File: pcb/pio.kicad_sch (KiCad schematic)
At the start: 32 parts, among them J11 GPA[0..3], J4 GPB[0..3], J5 GPB[4..7], J6 BTN[0..3], J7 GPA[4..7], U4 MCP23017T-E/ML

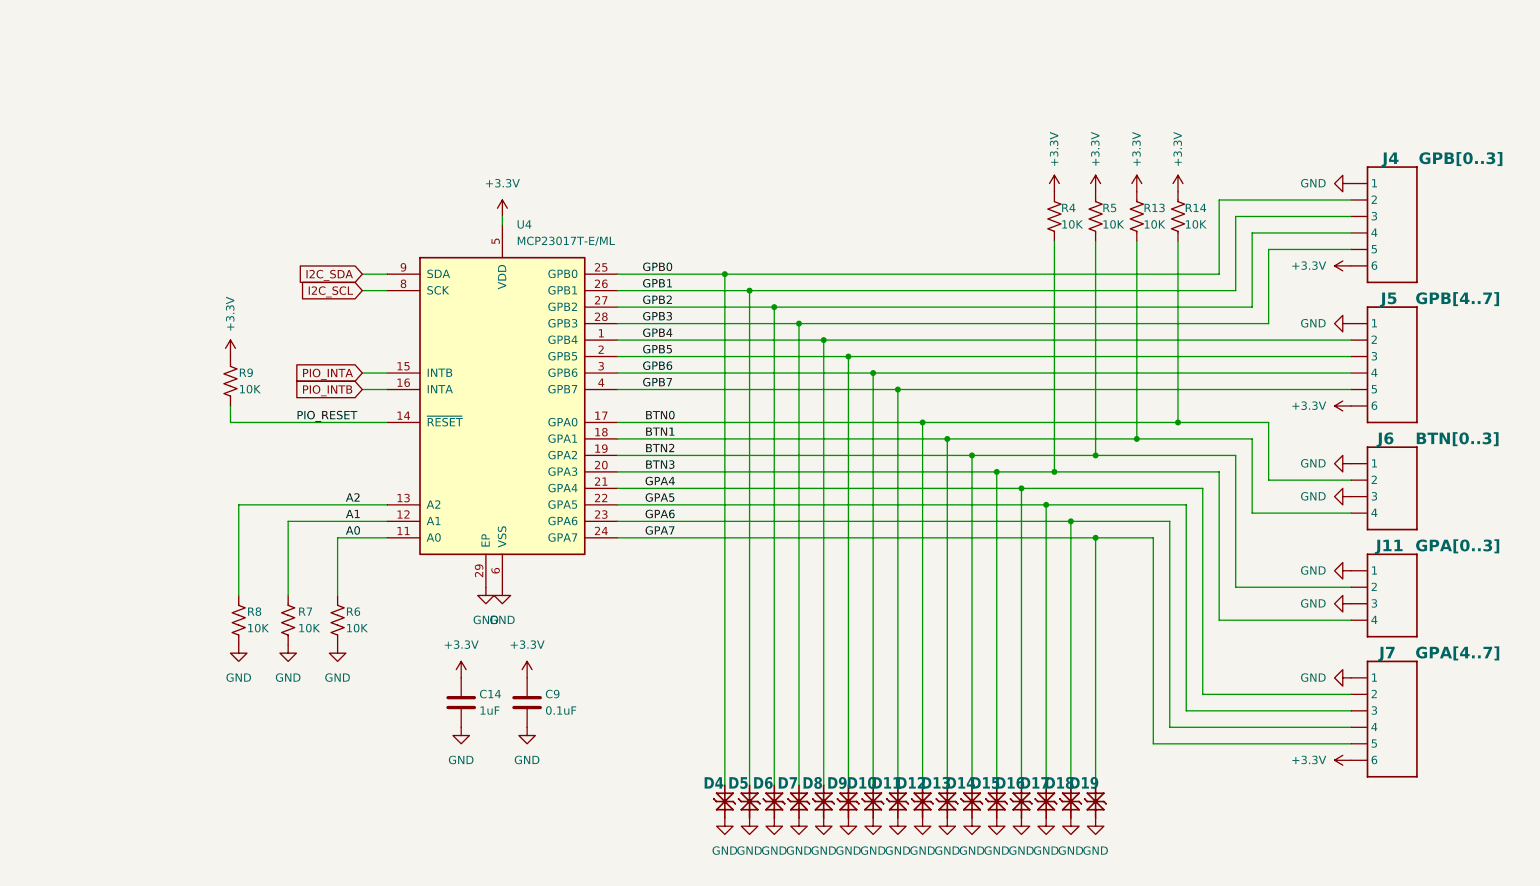
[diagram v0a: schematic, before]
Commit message: Cleaned up fab layer. Minor tweaks. Updated renders.
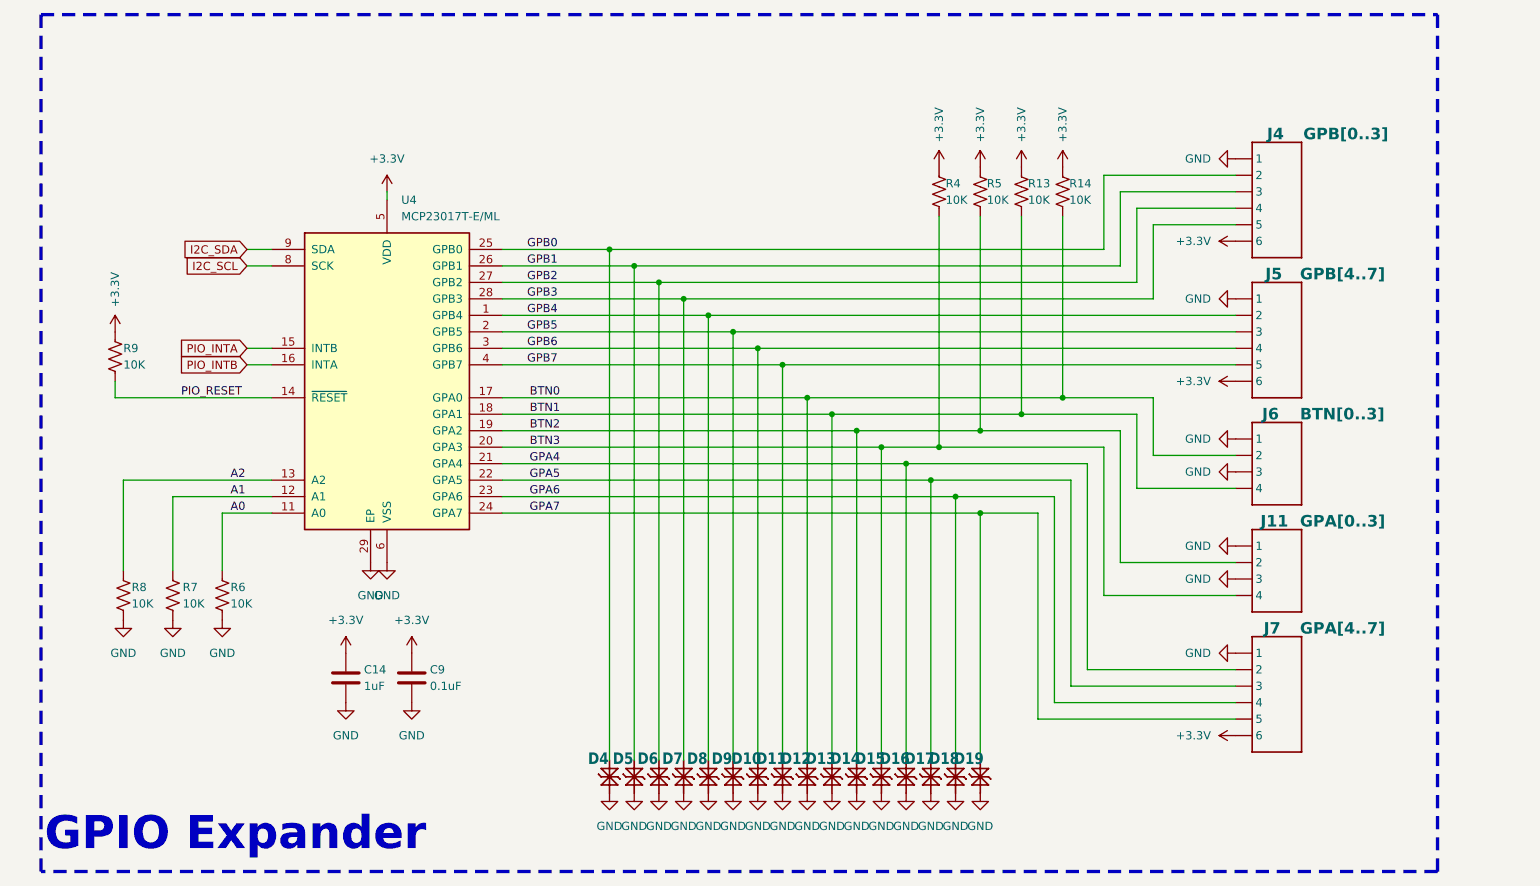
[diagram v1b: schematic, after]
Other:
- note added: "GPIO Expander"
- moved on the sheet: C14, C9, D10, D11, D12, D13, D14, D15, D16, D17, D18, D19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
